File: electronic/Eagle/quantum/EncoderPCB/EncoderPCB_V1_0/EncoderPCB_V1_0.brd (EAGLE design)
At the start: 38.1 x 68.2 mm, 15 parts, among them IC1 STM32F031K6T7

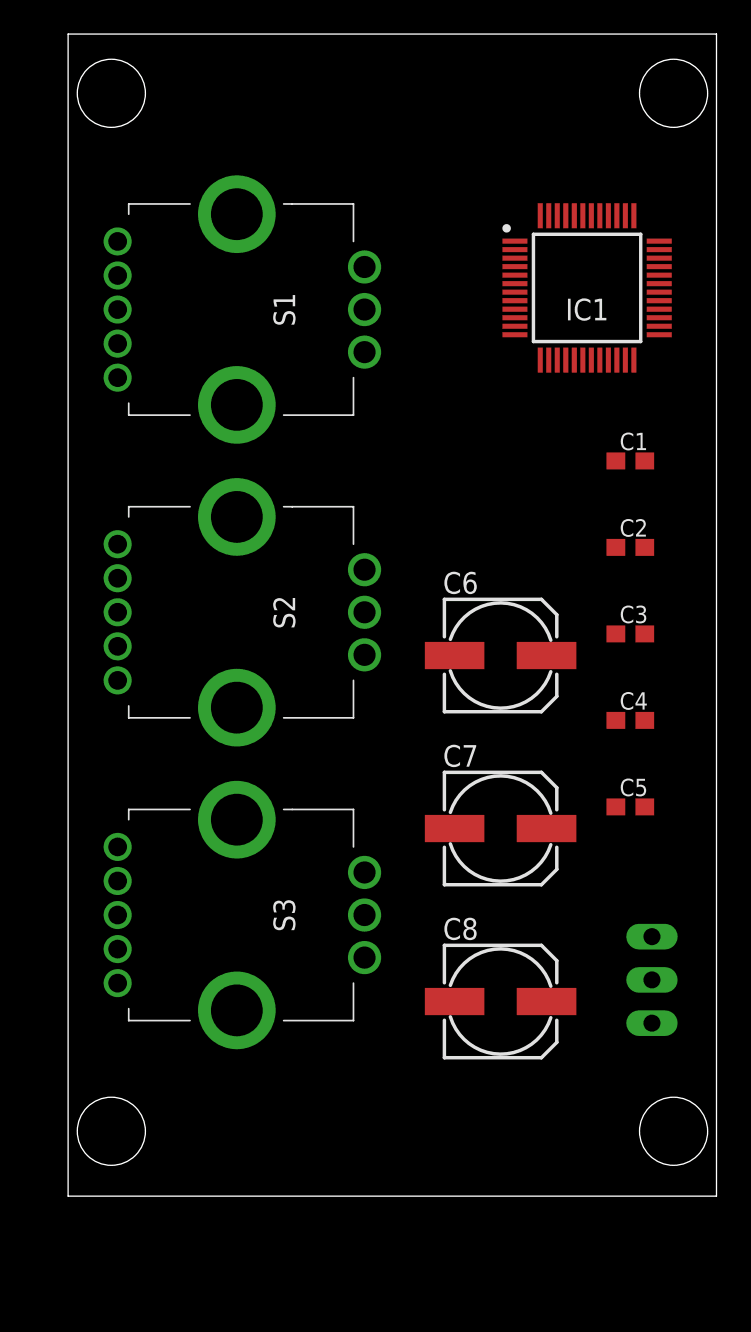
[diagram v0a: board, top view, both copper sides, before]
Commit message: Encoder PCB_V1_0 fertiggestellt
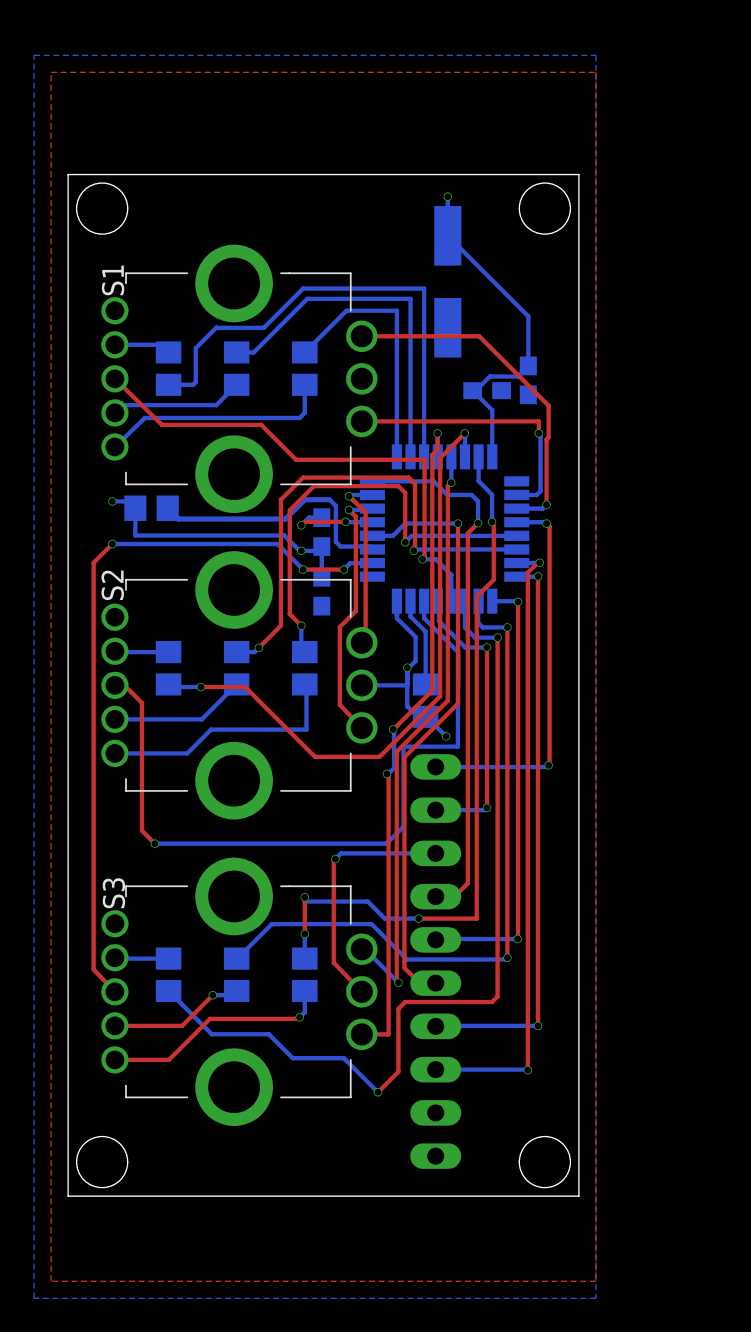
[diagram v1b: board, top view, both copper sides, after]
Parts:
- removed C5: 100nF, C_Sager_Bibliothek:C0603
- removed C6: 1µF, C_Sager_Bibliothek:153CLV-0605
- removed C7: 4,7µF, C_Sager_Bibliothek:153CLV-0605
- removed U$1, U$2, U$3: TPTHT, C_Sager_Bibliothek:THT_PIN
- added 3V1, GND, GND2, I2C1_SCL, I2C1_SDA, NRST, SWCLK, SWDIO, USART1_RX1, USART1_TX: TPTHT, C_Sager_Bibliothek:THT_PIN
- added R1, R11: 10k, C_Sager_Bibliothek:R0805
- added R10, R2, R3, R4, R5, R6, R7, R8, R9: (no value), C_Sager_Bibliothek:R0805
- IC1: value STM32F031K6T7 -> STM32F031K6T6; device C_Sager_Bibliothek:QFP50P900X900X160-48N -> C_Sager_Bibliothek:QFP80P900X900X160-32N
- moved C8 42.4 mm to (22.3, 53.7), flipped to the bottom, turned to 270 degrees
- moved C4 21.1 mm to (24.6, 47.3), flipped to the bottom
- moved C1 18.6 mm to (14.9, 39.0), flipped to the bottom, turned to 270 degrees
- moved C2 18.3 mm to (14.9, 35.5), flipped to the bottom, turned to 90 degrees
- moved IC1 16.4 mm to (22.1, 39.2), flipped to the bottom, turned to 180 degrees
- moved C3 16.0 mm to (27.0, 47.9), flipped to the bottom, turned to 90 degrees
- moved S3 4.51 mm to (10.0, 12.0)
- moved S2 4.29 mm to (10.0, 30.0)
- moved S1 4.07 mm to (10.0, 48.0)
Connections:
- new net ADRR.: IC1.3, R1.2
- new net BOOT_0: IC1.31, R11.2
- new net BUTTON_ENC1: IC1.28, S1.3
- new net BUTTON_ENC2: IC1.30, S2.3
- new net BUTTON_ENC3: IC1.2, S3.3
- new net B_ENC1: IC1.11, R4.1
- new net B_ENC2: IC1.14, R7.1
- new net B_ENC3: IC1.27, R10.1
- new net ENCODER1_A: IC1.18, S1.A1
- new net ENCODER1_B: IC1.19, S1.B1
- new net ENCODER2_A: IC1.6, S2.A1
- new net ENCODER2_B: IC1.7, S2.B1
- new net ENCODER3_A: IC1.12, S3.A1
- new net ENCODER3_B: IC1.13, S3.B1
- new net G_ENC1: IC1.10, R3.1
- new net G_ENC2: IC1.22, R6.1
- new net G_ENC3: IC1.26, R9.1
- new net I2C1_SCL: I2C1_SCL.P$1, IC1.29
- new net I2C1_SDA: I2C1_SDA.P$1, IC1.20
- new net N$10: R3.2, S1.2
- new net N$11: R5.2, S2.1
- new net N$12: R4.2, S1.4
- new net N$13: R6.2, S2.2
- new net N$14: R7.2, S2.4
- new net N$15: R8.2, S3.1
- new net N$16: R9.2, S3.2
- new net N$17: R10.2, S3.4
- new net N$9: R2.2, S1.1
- new net NRST: IC1.4, NRST.P$1
- new net R_ENC1: IC1.9, R2.1
- new net R_ENC2: IC1.21, R5.1
- new net R_ENC3: IC1.15, R8.1
- new net SWCLK: IC1.24, SWCLK.P$1
- new net SWDIO: IC1.23, SWDIO.P$1
- new net USART1_RX1: IC1.25, USART1_RX1.P$1
- new net USART1_TX: IC1.8, USART1_TX.P$1
- net +3V3: now also 3V1.P$1, IC1.17, IC1.5, S1.5, S2.5, S3.5; no longer C5.1, C6.+, C7.+, IC1.24, IC1.48, IC1.9
- net GND: now also GND.P$1, GND2.P$1, IC1.16, IC1.32, R1.1, R11.1, S1.C1, S2.C1, S3.C1; no longer C5.2, C6.-, C7.-, IC1.23, IC1.47, IC1.8
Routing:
- net GND: track 0.00 -> 65.7 mm, vias 0 -> 6
- net B_ENC3: track 0.00 -> 51.1 mm, vias 0 -> 2
- net BUTTON_ENC3: track 0.00 -> 43.3 mm, vias 0 -> 3
- net BUTTON_ENC2: track 0.00 -> 42.9 mm, vias 0 -> 1
- net R_ENC3: track 0.00 -> 42.3 mm, vias 0 -> 4
- net G_ENC3: track 0.00 -> 40.3 mm, vias 0 -> 2
- net ENCODER3_A: track 0.00 -> 39.6 mm, vias 0 -> 3
- net SWDIO: track 0.00 -> 36.9 mm, vias 0 -> 2
- net B_ENC2: track 0.00 -> 36.6 mm, vias 0 -> 2
- net ENCODER3_B: track 0.00 -> 35.2 mm, vias 0 -> 2
- net NRST: track 0.00 -> 34.9 mm, vias 0 -> 1
- net SWCLK: track 0.00 -> 33.7 mm, vias 0 -> 2
- net USART1_TX: track 0.00 -> 31.6 mm, vias 0 -> 1
- net BUTTON_ENC1: track 0.00 -> 29.7 mm, vias 0 -> 1
- net G_ENC2: track 0.00 -> 29.2 mm, vias 0 -> 2
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- added copper zone on layer 16, net +3V3
- added copper zone on layer 1, net GND
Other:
- board size 38.1 x 68.2 mm -> 30 x 60 mm
- board text added: "+3V3"
- board text added: "GND"
- board text added: "NRST"
- board text added: "RX"
- board text added: "SCL"
- board text added: "SDA"
- board text added: "SWCLK"
- board text added: "SWDIO"
- board text added: "TX"
